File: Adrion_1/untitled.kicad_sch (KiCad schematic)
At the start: 1 part, among them U2 STM32G474RET6

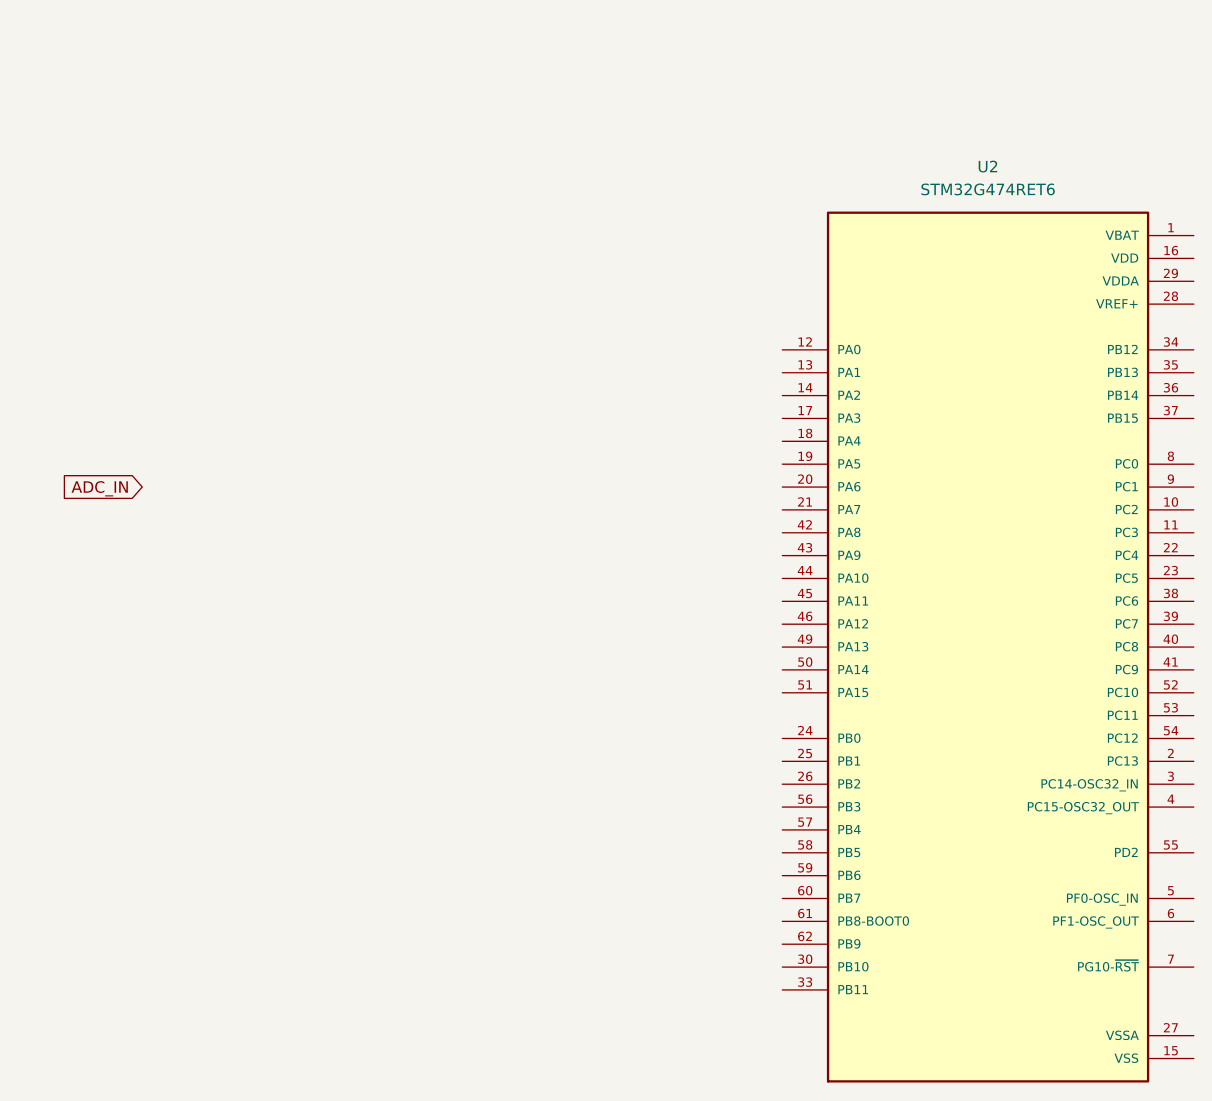
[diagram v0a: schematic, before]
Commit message: Modificaciones
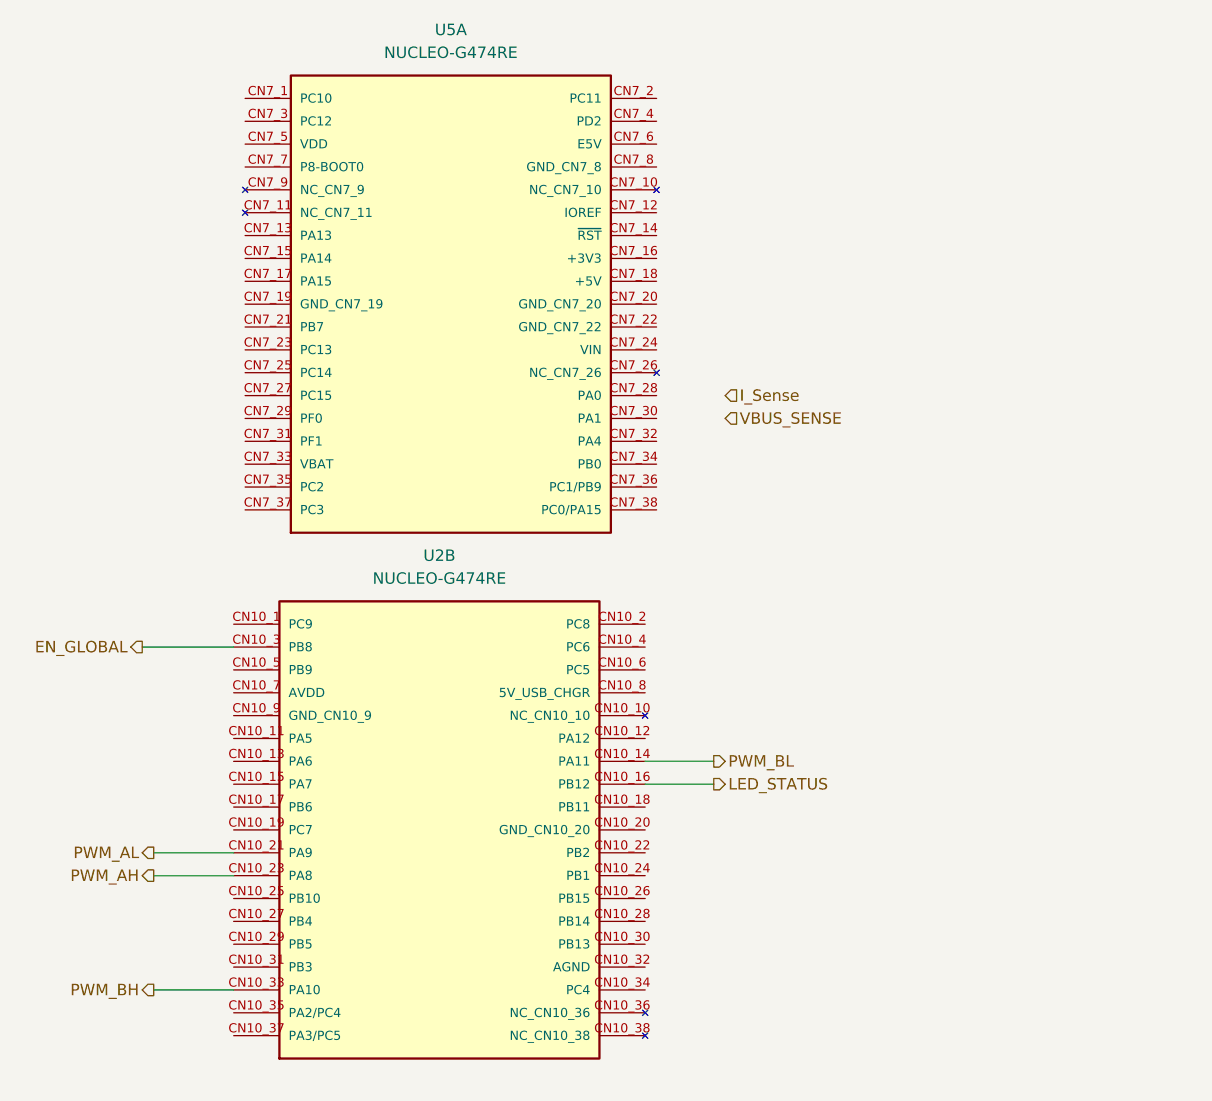
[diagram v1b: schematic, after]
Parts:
- removed U2: STM32G474RET6, STM32G474RET6:QFP50P1200X1200X160-64N, symbol STM32G474RET6:STM32G474RET6
- added U2, U5: NUCLEO-G474RE, NUCLEO-G474RE:MODULE_NUCLEO-G474RE, symbol NUCLEO-G474RE_3p:NUCLEO-G474RE
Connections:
- new net EN_GLOBAL: U2.CN10_3 (PB8)
- new net LED_STATUS: U2.CN10_16 (PB12)
- new net PWM_AH: U2.CN10_23 (PA8)
- new net PWM_AL: U2.CN10_21 (PA9)
- new net PWM_BH: U2.CN10_33 (PA10)
- new net PWM_BL: U2.CN10_14 (PA11)
